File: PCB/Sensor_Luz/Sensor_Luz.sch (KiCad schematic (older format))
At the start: 12 parts, among them J1 Conn_02x20_Odd_Even, J2 Conn_02x20_Odd_Even, J3 Conn_01x02_Male, J4 Conn_01x04_Female, J5 Conn_01x02_Male, J6 Conn_01x06_Female, J7 Conn_01x02_Male, Q1 BC817

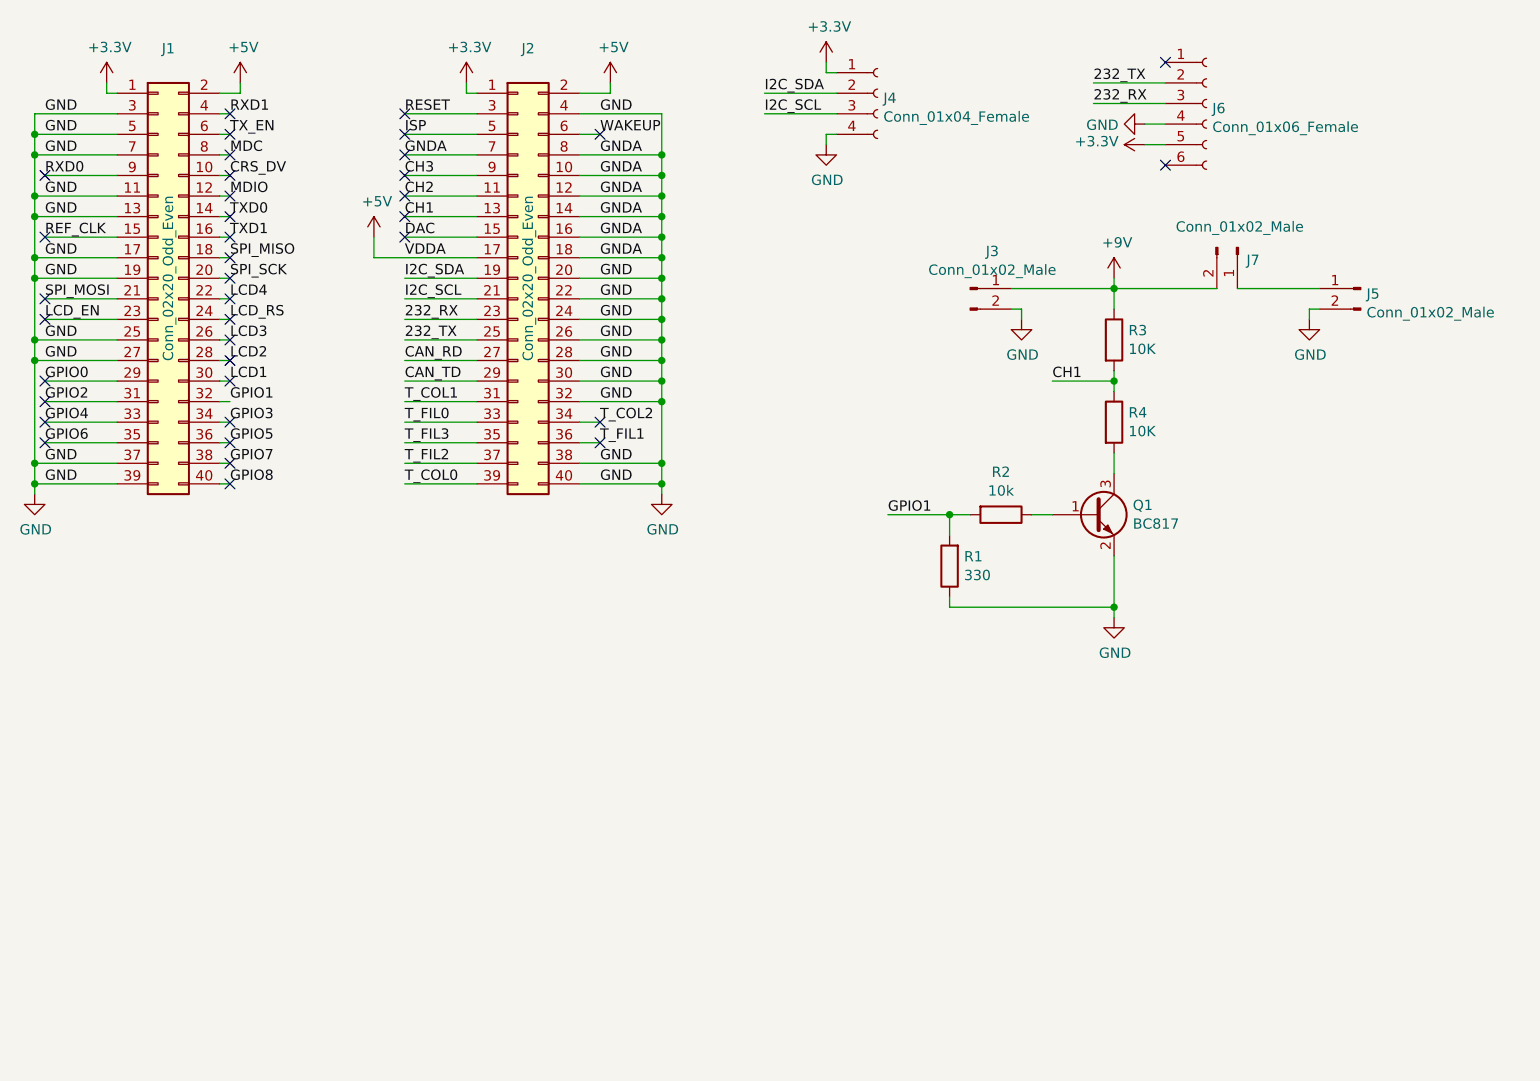
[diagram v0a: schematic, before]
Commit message: PCB actualizado
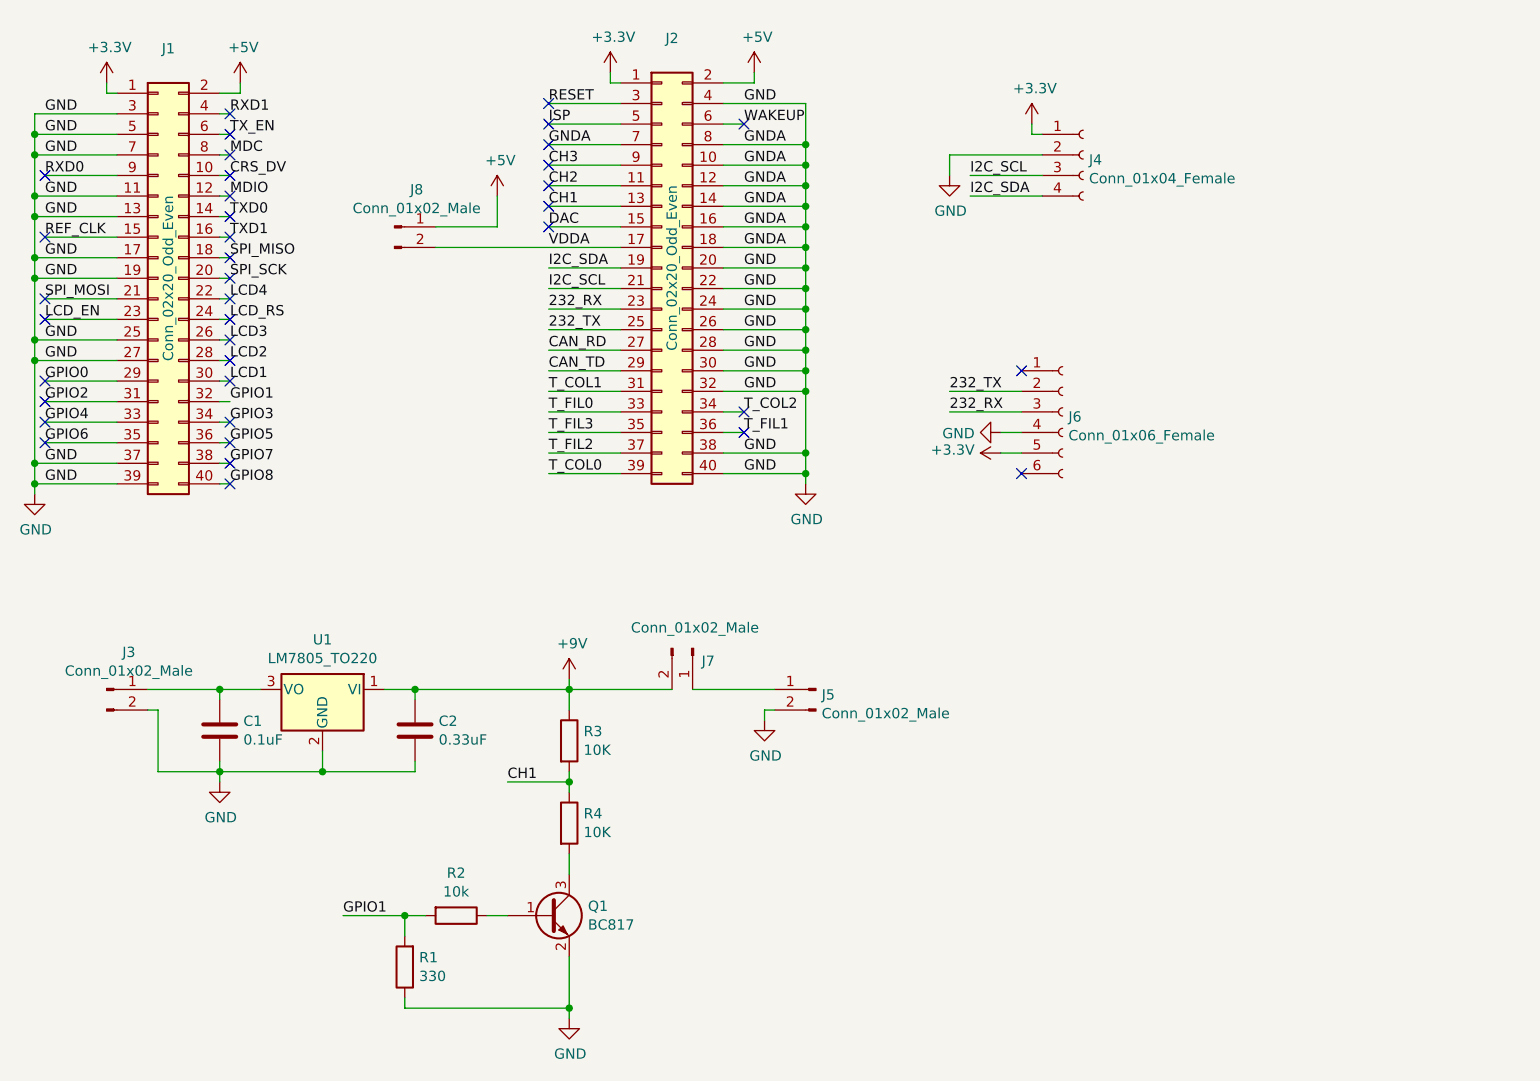
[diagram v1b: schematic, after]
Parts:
- added C1: 0.1uF, Capacitor_THT:C_Disc_D5.0mm_W2.5mm_P2.50mm, symbol Device:C
- added C2: 0.33uF, Capacitor_THT:C_Disc_D5.0mm_W2.5mm_P2.50mm, symbol Device:C
- added J8: Conn_01x02_Male, Connector_PinSocket_2.54mm:PinSocket_1x02_P2.54mm_Vertical, symbol Connector:Conn_01x02_Male
- added U1: LM7805_TO220, Package_TO_SOT_THT:TO-220-3_Vertical, symbol Regulator_Linear:LM7805_TO220
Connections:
- net +5V: now also J8.1 (Pin_1); no longer J2.17 (Pin_17)
- net +9V: now also C2.1, U1.1 (VI); no longer J3.1 (Pin_1)
- net GND: now also J4.2 (Pin_2), C1.2, C2.2, U1.2 (GND); no longer J4.4 (Pin_4)
- net I2C_SDA: now also J4.4 (Pin_4); no longer J4.2 (Pin_2)
- new net: C1.1, J3.1 (Pin_1), U1.3 (VO)
- new net VDDA: J2.17 (Pin_17), J8.2 (Pin_2)
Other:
- moved on the sheet: J2, J3, J4, J5, J6, J7, Q1, R1, R2, R3, R4
